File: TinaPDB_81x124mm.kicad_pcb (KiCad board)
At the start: 2 copper layers, 119.6 x 57.4 mm, 28 parts, among them J1 Main Computer (Jetson), J10 Drive 1, J11 Drive 2, J12 Drive 3, J13 Drive 4, J14 Digger 1, J15 Digger 2, J16 Bucket 1, J17 Bucket 2, J18 MAux 1, J19 Conn_02x02_Counter_Clockwise, J2 IMU, J3 Localization, J4 Second Computer, J5 Aux 1, J6 Aux 2, J7 Aux 3, J8 Main Button, J9 JM Button, K1 FINDER-36.11-4301, K2 FINDER-36.11-4301

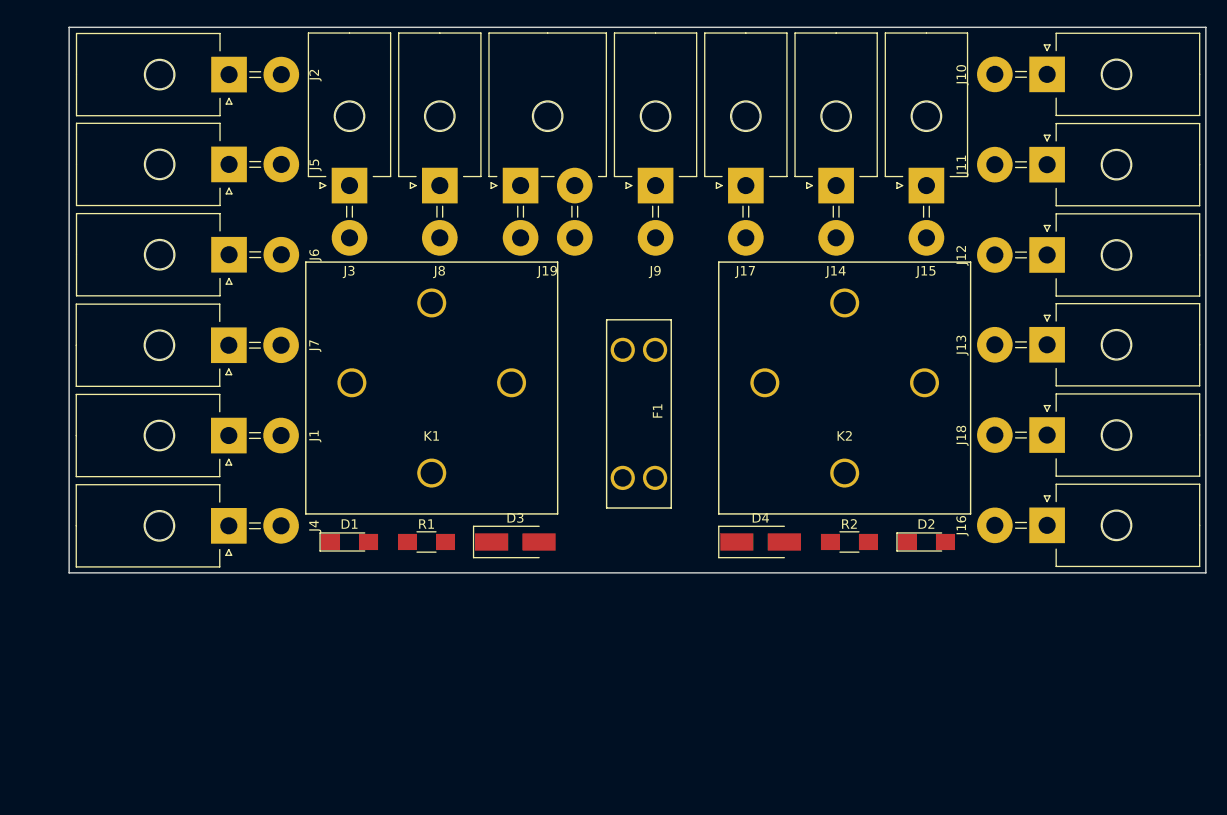
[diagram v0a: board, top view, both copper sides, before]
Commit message: Made layout
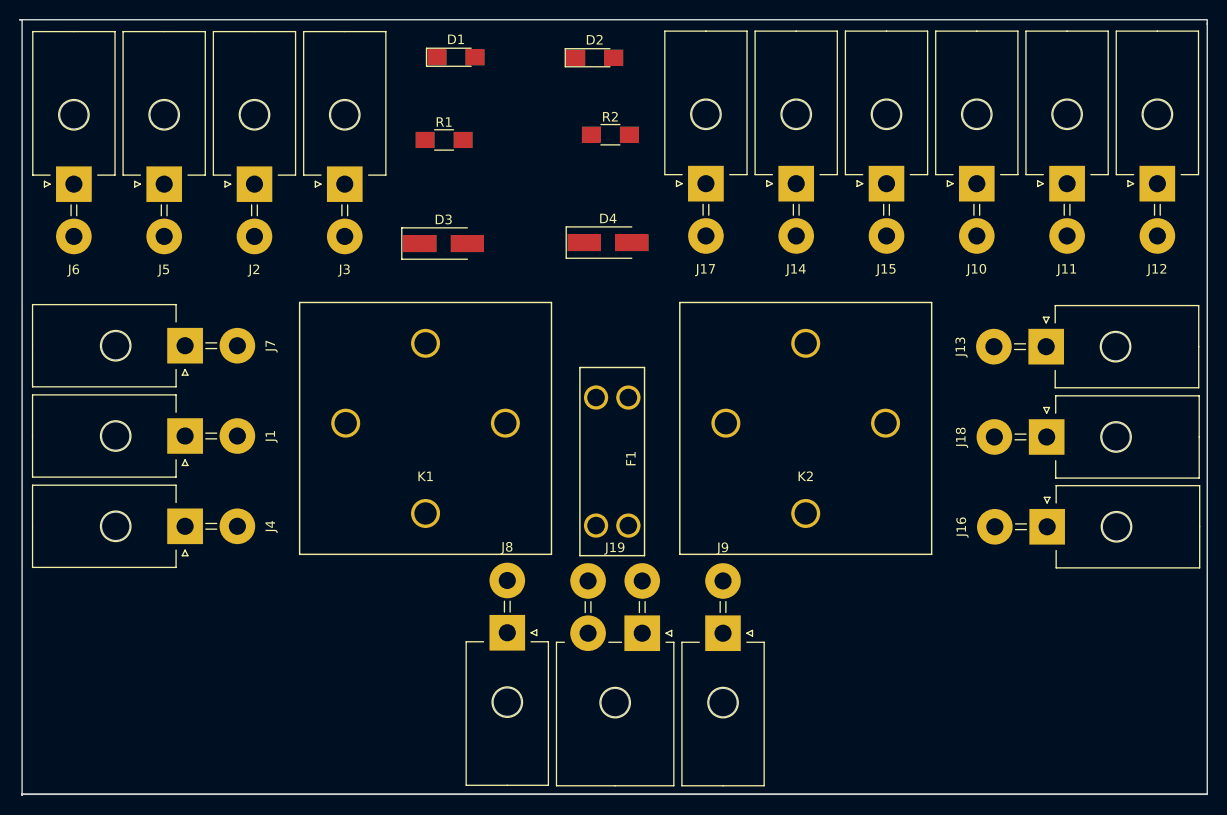
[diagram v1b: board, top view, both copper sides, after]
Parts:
- moved D2 61.8 mm to (178.5, 68.0)
- moved D1 52.2 mm to (163.9, 68.0)
- moved R2 49.7 mm to (180.2, 76.1)
- moved J19 48.8 mm to (183.5, 128.6), turned to 180 degrees
- moved J9 47.6 mm to (192.0, 128.6), turned to 180 degrees
- moved J8 47.6 mm to (169.3, 128.5), turned to 180 degrees
- moved R1 42.3 mm to (162.7, 76.7)
- moved D4 35.4 mm to (179.9, 87.5)
- moved D3 32.3 mm to (162.6, 87.5)
- moved J6 17.9 mm to (123.7, 81.3), turned to 0 degrees
- moved J12 13.8 mm to (237.7, 81.2), turned to 0 degrees
- moved J10 13.7 mm to (218.7, 81.2), turned to 0 degrees
- moved J2 11.8 mm to (142.7, 81.3), turned to 0 degrees
- moved J5 7.13 mm to (133.2, 81.3), turned to 0 degrees
- moved K2 5.91 mm to (200.7, 107.0)
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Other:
- board size 119.6 x 57.4 mm -> 124.9 x 81.6 mm
